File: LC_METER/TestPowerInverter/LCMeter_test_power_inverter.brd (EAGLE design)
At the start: 60 x 28 mm, 34 parts, among them IC10 MC34063, T1 H772, X1 VCC_IN, X2 GND, X3 +5V_STAB, X4 +7V, X5 -7V, X6 GND

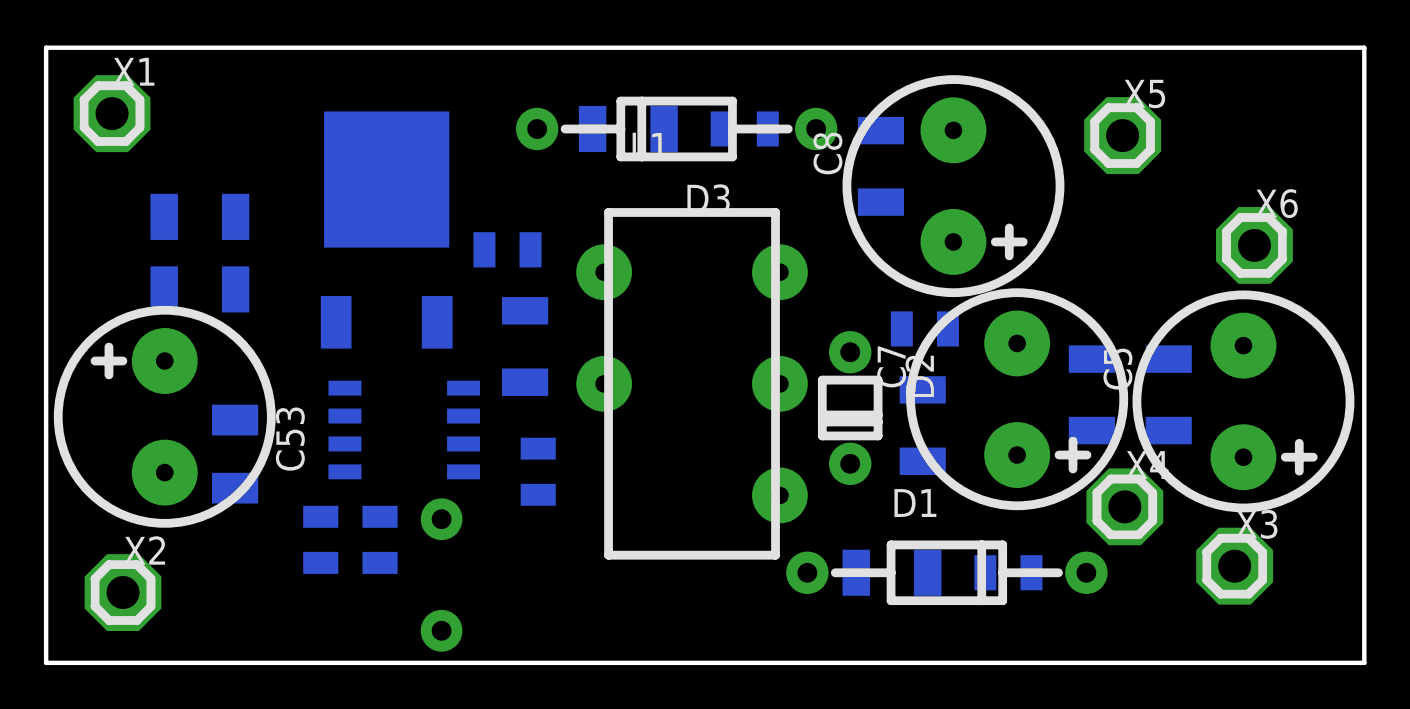
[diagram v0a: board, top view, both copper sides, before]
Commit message: LC meter test power supply inverter. almost routed
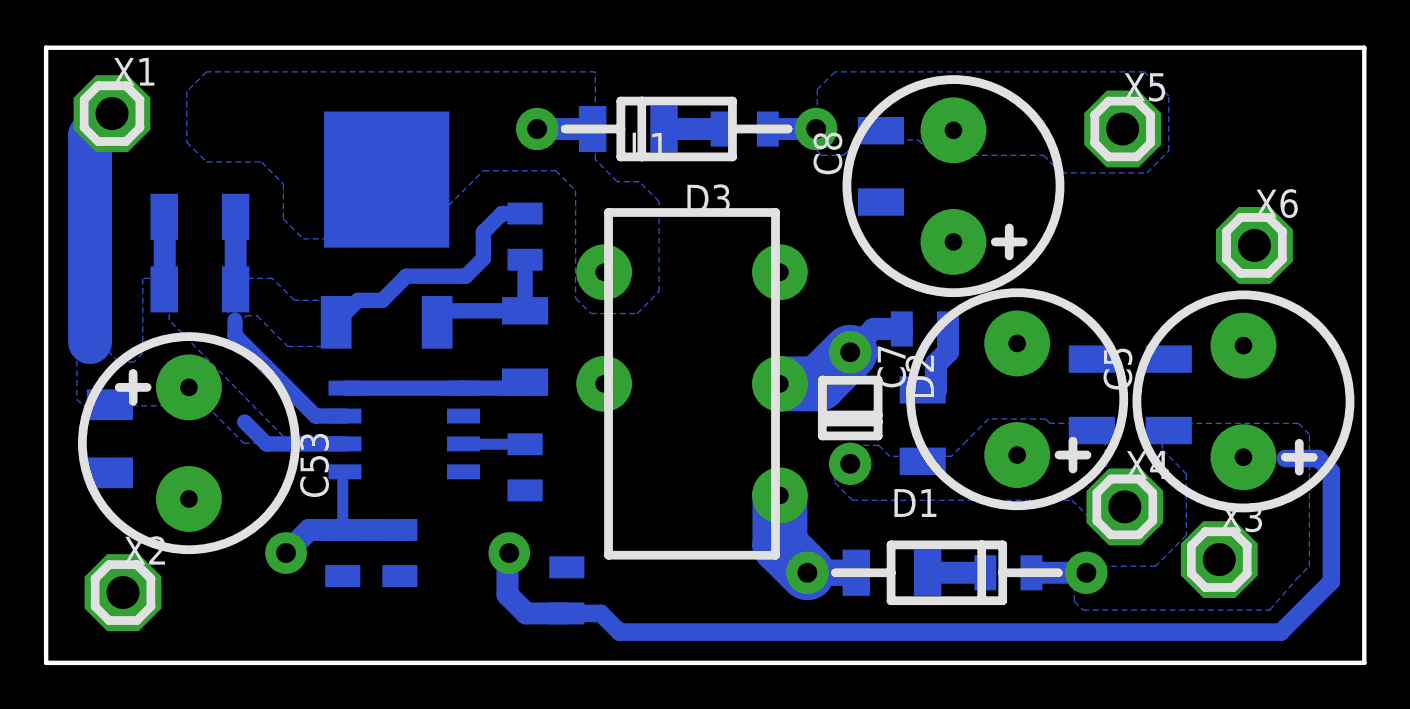
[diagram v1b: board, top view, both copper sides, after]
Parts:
- added C10: 0.1uF, __MyCommonLib1:RSMD_0805
- R84: device __MyCommonLib1:R0204 -> __MyCommonLib1:R0207
- moved C54 5.74 mm to (2.90, 10.2)
- moved R84 2.24 mm to (16.0, 5.00), turned to 180 degrees
- moved C53 1.63 mm to (6.50, 10.0)
- moved R7 1.17 mm to (13.5, 5.00)
- moved R85 1.08 mm to (16.1, 5.00)
- moved R2 1.00 mm to (21.8, 19.4), turned to 90 degrees
- moved X3 0.76 mm to (53.4, 4.70)
- moved C55 0.63 mm to (21.8, 8.90)
- moved X5 0.30 mm to (49.0, 24.3)
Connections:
- net +5V_STAB: now also C10.PAD_1
- net GND: now also C10.PAD_0
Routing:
- net +5V_STAB: track 0.00 -> 50.9 mm
- net N$3: track 0.00 -> 21.9 mm
- net VCC_IN: track 0.00 -> 19.1 mm
- net N$139: track 0.00 -> 8.36 mm
- net N$133: track 0.00 -> 8.31 mm
- net N$8: track 0.00 -> 6.59 mm
- net N$2: track 0.00 -> 6.54 mm
- net N$7: track 0.00 -> 6.26 mm
- net N$1: track 0.00 -> 3.64 mm
- net N$135: track 0.00 -> 2.82 mm
- net N$5: track 0.00 -> 2.62 mm
- net N$10: track 0.00 -> 2.62 mm
- net N$4: track 0.00 -> 2.52 mm
- net -7V: track 0.00 -> 2.20 mm
- added copper zone on layer 16, net +5V_STAB
- added copper zone on layer 16, net +7V
- added copper zone on layer 16, net -7V
- added copper zone on layer 16, net N$3
- added copper zone on layer 16, net N$4
- added copper zone on layer 16, net VCC_IN
